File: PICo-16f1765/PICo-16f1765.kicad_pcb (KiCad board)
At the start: 2 copper layers, 20.3 x 67.3 mm, 26 parts, among them IC1 PIC16F1765-I_P, IC2 CH340K, J1 Conn_01x06_Female, J2 Conn_01x09_Female, J3 Conn_01x09_Female, J4 USB_B_Micro, SW1 SW_Push, SW2 SW_Push, U1 LM1117-3.3, U2 LM1117S50TR_SOT223, Y1 Crystal

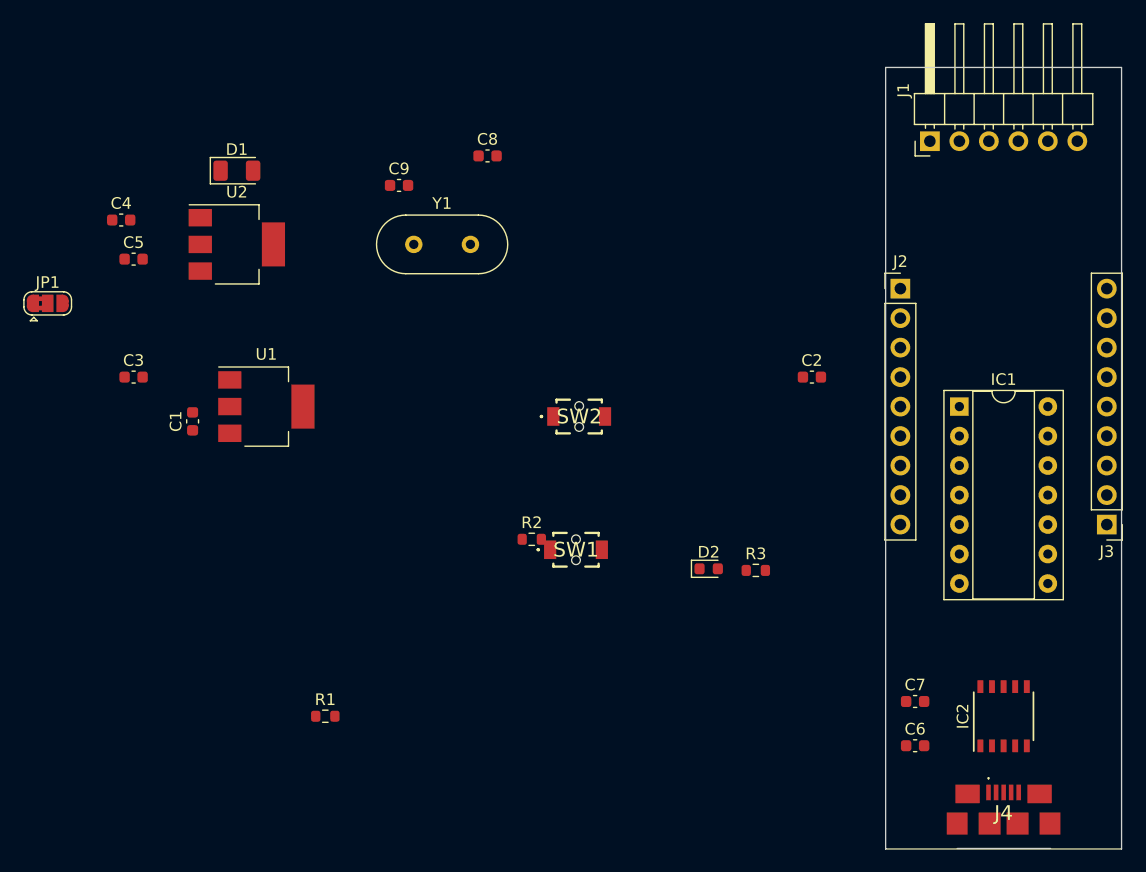
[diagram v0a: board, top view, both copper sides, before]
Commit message: kansei
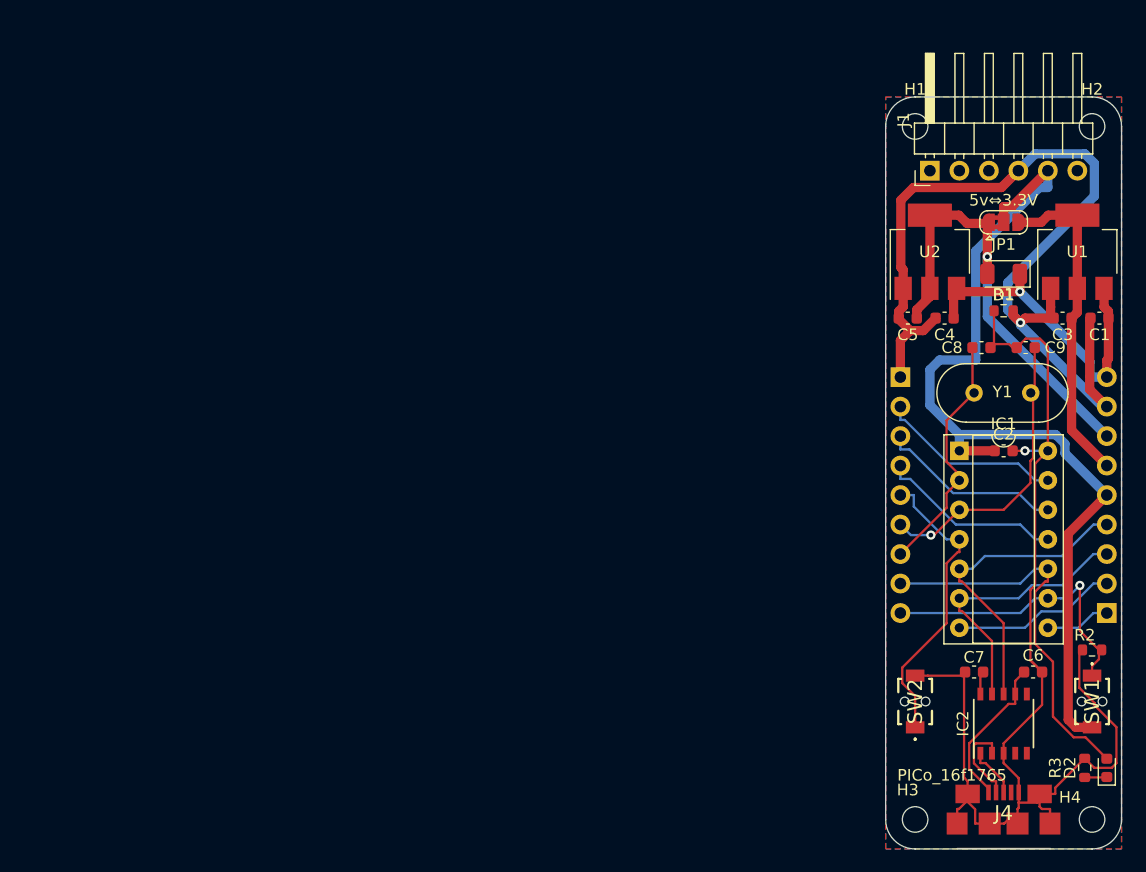
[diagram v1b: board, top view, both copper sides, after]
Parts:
- added H1: MountingHole, MountingHole:MountingHole_2.2mm_M2, F.Cu at (-3.81, -14.0)
- added H2: MountingHole, MountingHole:MountingHole_2.2mm_M2, F.Cu at (11.4, -14.0)
- added H3: MountingHole, MountingHole:MountingHole_2.2mm_M2, F.Cu at (-3.81, 45.7)
- added H4: MountingHole, MountingHole:MountingHole_2.2mm_M2, F.Cu at (11.4, 45.7)
- J2, J3: moved to B.Cu
- moved JP1 82.6 mm to (3.81, -5.71)
- moved C3 80.2 mm to (8.89, 2.54), turned to 180 degrees
- moved C1 78.6 mm to (12.1, 2.54), turned to 180 degrees
- moved C4 71.4 mm to (-1.27, 2.54), turned to 180 degrees
- moved U1 71.1 mm to (10.2, -3.17), turned to 90 degrees
- moved R1 68.1 mm to (3.81, 1.91)
- moved C5 66.9 mm to (-4.45, 2.54), turned to 180 degrees
- moved D1 66.6 mm to (3.81, -1.27), turned to 180 degrees
- moved U2 59.7 mm to (-2.54, -3.17), turned to 90 degrees
- moved C9 55.8 mm to (5.71, 5.08), turned to 180 degrees
- moved Y1 49.9 mm to (1.27, 8.98)
- moved R2 49.2 mm to (11.4, 31.1), turned to 180 degrees
- moved SW1 46.3 mm to (11.4, 35.6), turned to 270 degrees
- moved C8 45.6 mm to (1.91, 5.08)
- moved D2 38.3 mm to (12.7, 41.3), turned to 90 degrees
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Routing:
- net GND: track 0.00 -> 106.3 mm, vias 0 -> 1
- net GNDPWR: track 0.00 -> 80.5 mm, vias 0 -> 1
- net VCC: track 0.00 -> 79.5 mm
- net +5V: track 0.00 -> 39.1 mm, vias 0 -> 1
- net /RC0: track 0.00 -> 33.3 mm
- net /Vin: track 0.00 -> 28.9 mm, vias 0 -> 1
- net +3V3: track 0.00 -> 28.6 mm
- net /RC5: track 0.00 -> 26.8 mm
- net /RA4: track 0.00 -> 26.2 mm, vias 0 -> 1
- net /RA3_MCLR: track 0.00 -> 26.0 mm
- net /RC1: track 0.00 -> 25.4 mm, vias 0 -> 1
- net /RC4: track 0.00 -> 23.8 mm
- net /RA5: track 0.00 -> 21.4 mm
- net /RA1_ICSPCLK: track 0.00 -> 16.0 mm
- net /RA0_ICSPDAT: track 0.00 -> 16.0 mm
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- added copper zone on B.Cu, net GND
- added copper zone on F.Cu, net GND
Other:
- board size 20.3 x 67.3 mm -> 20.3 x 64.8 mm
- net class Default: trace_width 0.25 -> 0.2
- net class Power added: clearance 0.2, trace_width 0.8, via_dia 0.8, via_drill 0.4
- board text added: "5v⇔3.3V"
- board text added: "PICo_16f1765"
